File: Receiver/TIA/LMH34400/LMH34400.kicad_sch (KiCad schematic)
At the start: 24 parts, among them J1 TEST, J2 PD IN, J3 Vout, J4 N_EN, J5 N_ALC, J6 OUT, U1 LMH34400

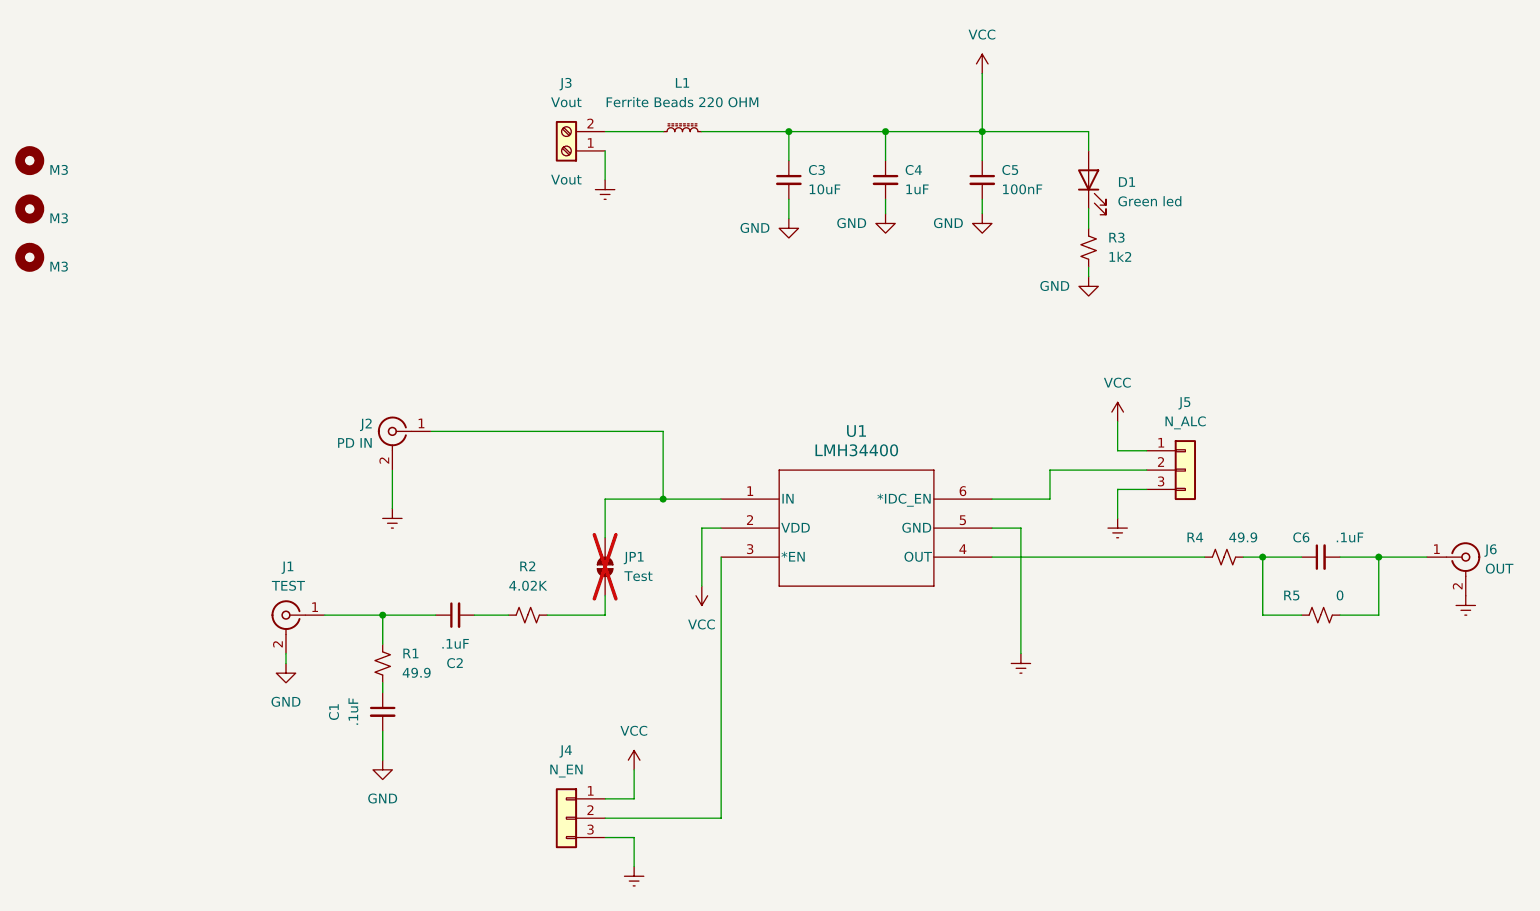
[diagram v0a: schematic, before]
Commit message: LTC6268-10 first version
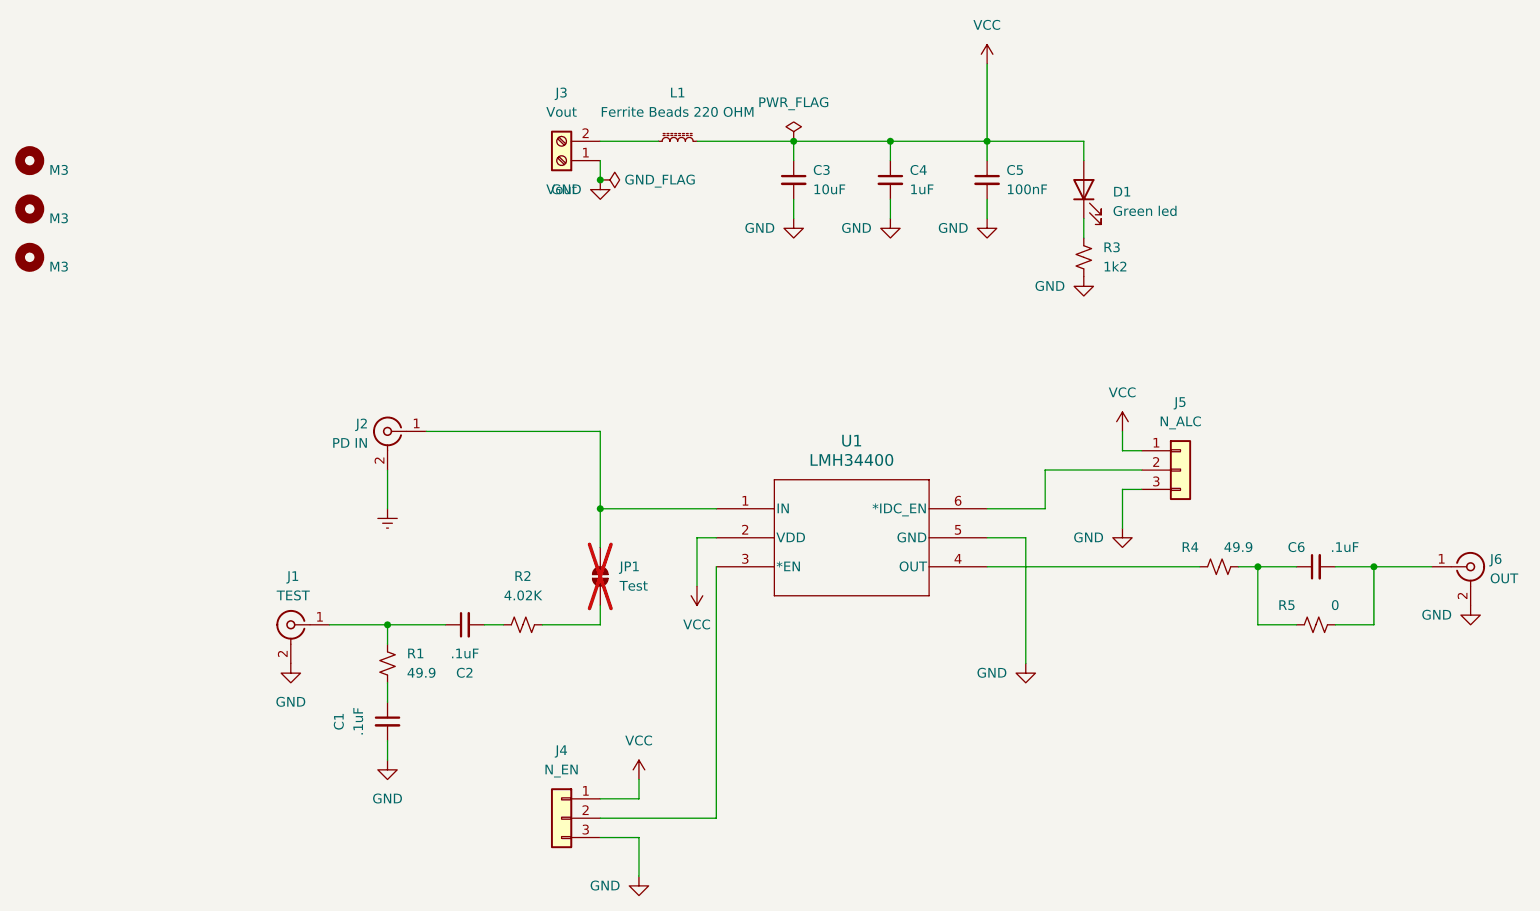
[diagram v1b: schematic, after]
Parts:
- D1: footprint LumiCom_TIA:LEDC1608X80N -> LED_SMD:LED_0603_1608Metric
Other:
- moved on the sheet: C1, C2, C3, C4, C5, C6, D1, J1, J2, J3, J4, J5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

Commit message: LMH3440 fixed
LMH3440 fixed
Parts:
- R3: Manufacturer Part Number CRCW08051K20FKEAC -> CRCW06031K20FKEA; Mouser Part Number 71-CRCW08051K20FKEAC -> 71-CRCW0603-1.2K-E3
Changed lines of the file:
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@@
 			)
 		)
-		(property "Datasheet" "https://www.vishay.com/doc?28773"
+		(property "Datasheet" "https://www.vishay.com/doc?20035"
 			(at 195.58 68.58 0)
 			(effects
@@
 			)
 		)
-		(property "Description" "1/8Watt 1.2Kohms 1% Commercial Use"
+		(property "Description" " Thick Film Resistors - SMD 1/10watt 1.2Kohms 1% 0603"
 			(at 195.58 68.58 0)
 			(effects
@@
 			)
 		)
-		(property "Manufacturer Part Number" "CRCW08051K20FKEAC"
+		(property "Manufacturer Part Number" " CRCW06031K20FKEA "
 			(at 195.58 68.58 0)
 			(effects
@@
 			)
 		)
-		(property "Mouser Part Number" " 71-CRCW08051K20FKEAC "
+		(property "Mouser Part Number" " 71-CRCW0603-1.2K-E3 "
 			(at 195.58 68.58 0)
 			(effects
